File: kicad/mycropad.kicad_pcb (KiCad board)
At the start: 2 copper layers, 116.2 x 64.8 mm, 33 parts, among them SW1 SW_Push, SW2 SW_Push, SW3 SW_Push, SW4 SW_Push, SW5 SW_Push, SW6 SW_Push, SW7 SW_Push, SW8 SW_Push, U1 Pico, U2 SN74AHCT125N

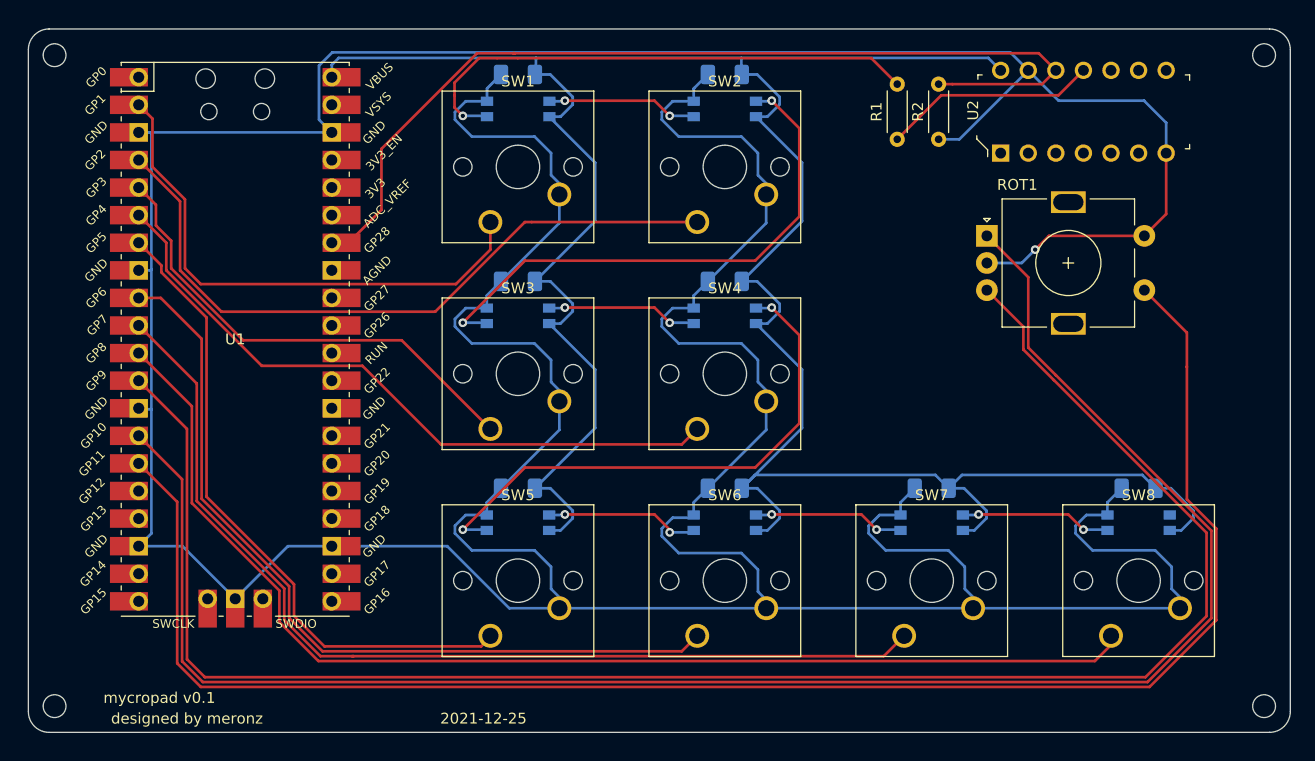
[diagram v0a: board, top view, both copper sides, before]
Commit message: mycropad v0.2 started.
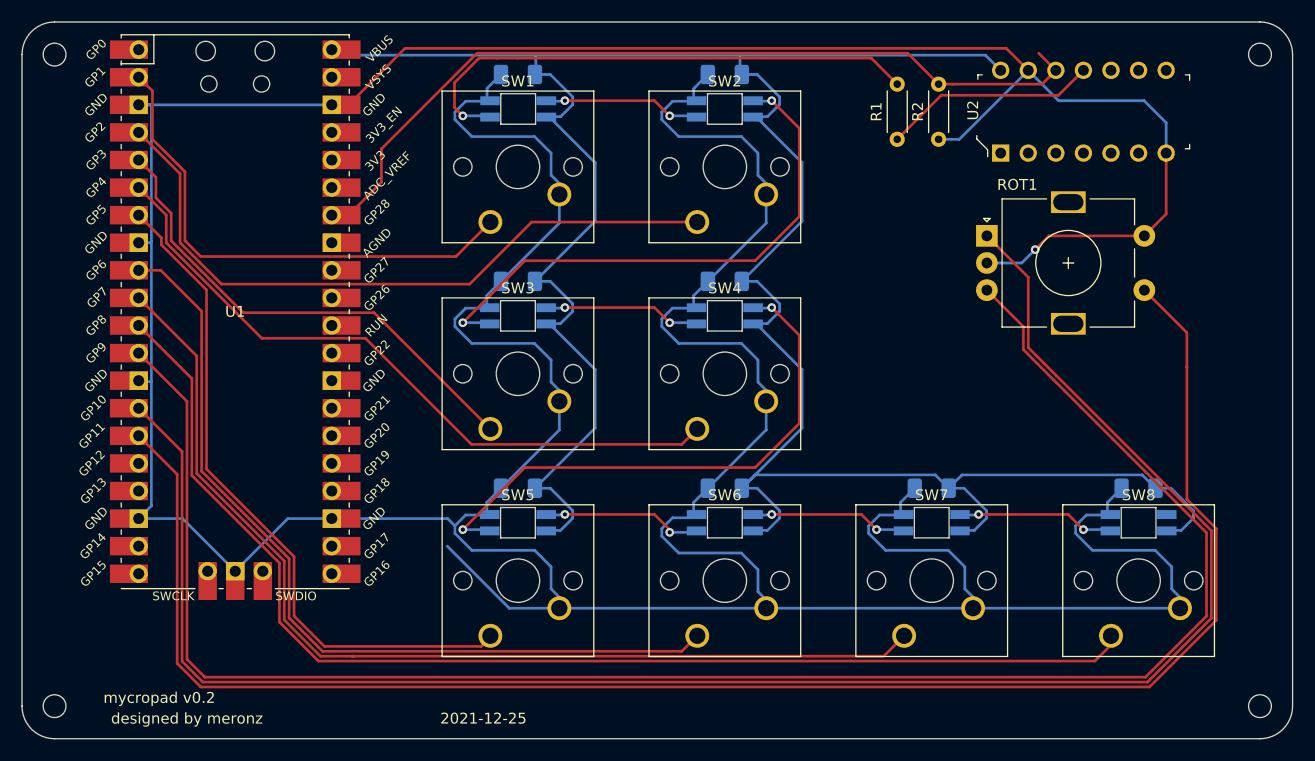
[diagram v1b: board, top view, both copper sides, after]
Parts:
- D1, D2, D3, D4, D5, D6, D7, D8: footprint mycropad:LED_SK6812MINI-E_REV02_PLCC4_3.5x3.5mm_P1.75mm -> mycropad:LED_SK6812MINI-E_REV02_PLCC4_3.5x3.5mm_P1.75mm___V2
- moved U1 2.54 mm to (90.8, 89.5)
- moved REF** 0.38 mm to (185.2, 65.9)
- moved REF** 0.38 mm to (185.2, 125.9)
- moved REF** 0.06 mm to (74.2, 65.9)
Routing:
- net GPIO28: track 89.3 -> 78.6 mm
- net GND: track 493.5 -> 488.4 mm
- net GPIO5: track 60.0 -> 62.6 mm
- net GPIO11: track 152.1 -> 154.7 mm
- net GPIO9: track 162.9 -> 165.4 mm
- net GPIO6: track 75.8 -> 78.4 mm
- net GPIO10: track 164.2 -> 166.7 mm
- net GPIO1: track 49.4 -> 46.9 mm
- net GPIO8: track 109.7 -> 112.2 mm
- net GPIO7: track 92.1 -> 94.6 mm
- net GPIO3: track 44.2 -> 45.2 mm
- net GPIO2: track 64.4 -> 63.3 mm
- net GPIO4: track 62.3 -> 63.3 mm
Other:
- board size 116.2 x 64.8 mm -> 117 x 66 mm
- board text added: "mycropad v0.2"
- board text removed: "mycropad v0.1"
